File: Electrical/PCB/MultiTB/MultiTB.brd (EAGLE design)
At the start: 9 parts, among them U2 TB6612FNG

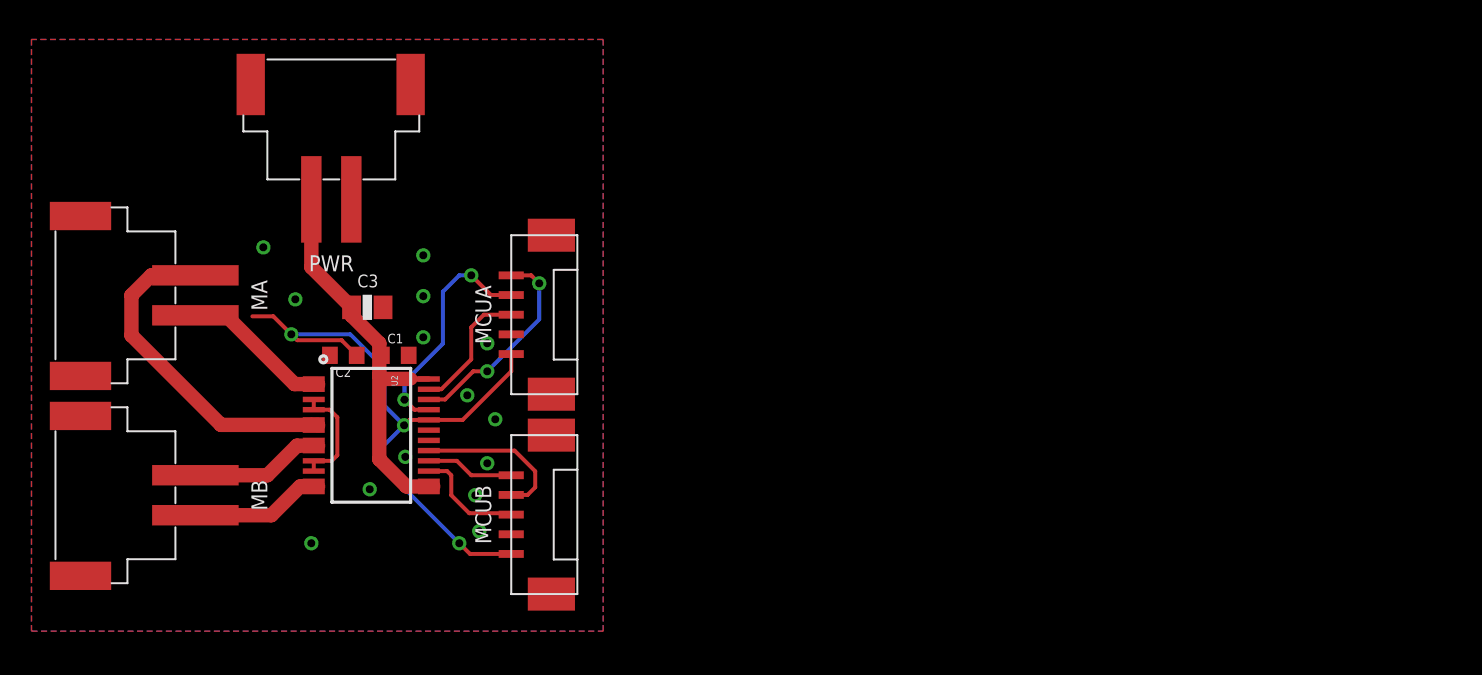
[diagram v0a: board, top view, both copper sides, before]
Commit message: PCB Batch #1
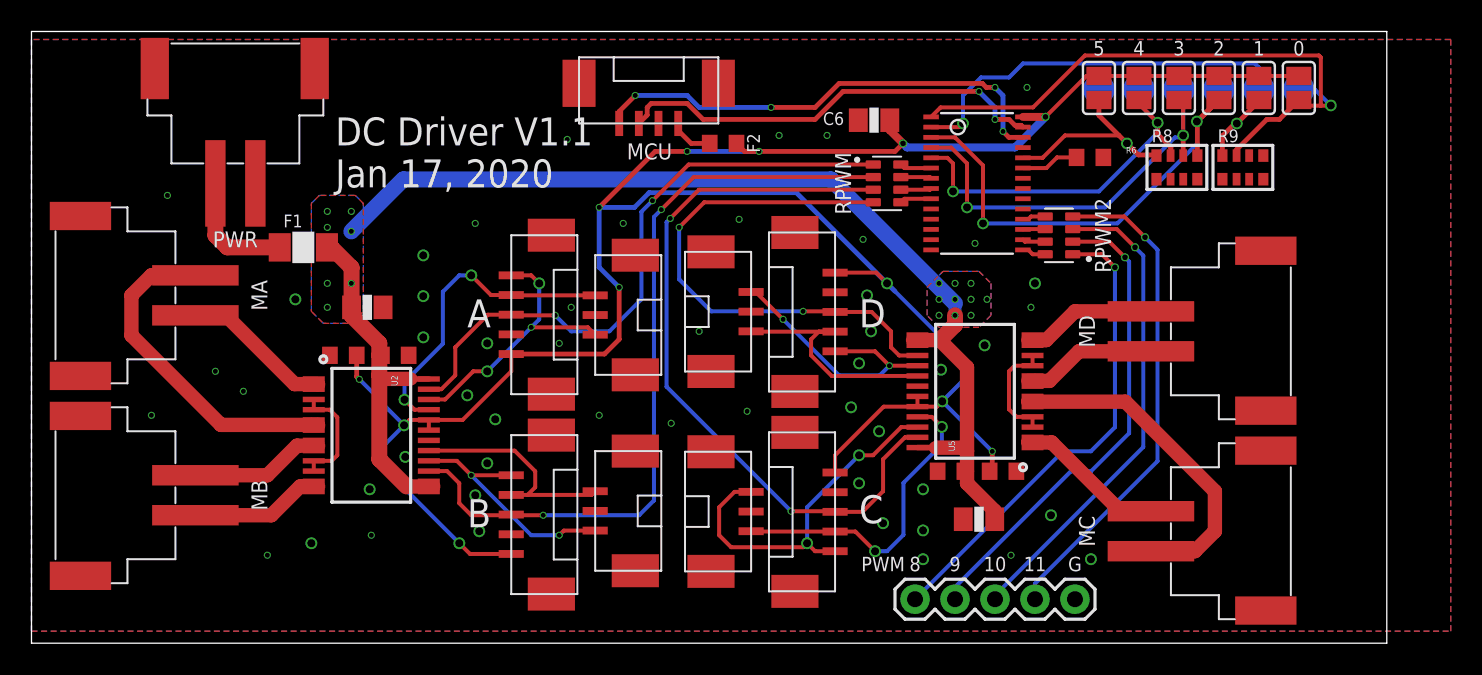
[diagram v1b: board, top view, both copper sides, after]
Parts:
- added C11, C12: 0.1uF, Scott-Electrical:0603
- added C13, C6: 10uF, Scott-Electrical:0805
- added F1: 7A, Scott-Electrical:1206
- added F2: 2A, Scott-Electrical:0603
- added J1: (no value), SparkFun-Connectors:1X05
- added MACTRL, MBCTRL, MCCTRL, MDCTRL: JST_1.25_3P, Scott-Connectors:JST1.25_3P
- added MC, MD: JST_XH_2.54_2P, Scott-Connectors:JST_XH_2.54_2P
- added MCU: JST_1.25_4P, Scott-Connectors:JST1.25_4P
- added MCUC, MCUD: JST_1.25_5P, Scott-Connectors:JST1.25_5P
- added R6: 10K, Scott-Electrical:0603
- added R8, R9: 10K, microbuilder:RESPACK_4X0603
- added RPWM, RPWM2: 330, Scott-Electrical:RESCAF80P320X160X60-8N
- added SJ_A12, SJ_A13, SJ_A14, SJ_A15, SJ_A16, SJ_A17: (no value), microbuilder:SOLDERJUMPER_REFLOW_NOPASTE
- added TP13, TP14, TP15, TP16, TP17, TP18: (no value), microbuilder:TESTPOINT_ROUND_2MM
- added U4: PCA9685, microbuilder:TSSOP28
- added U5: TB6612FNG, SparkFun-IC-Special-Function:SSOP24
- moved PWR 6.18 mm to (1.52, 30.2)
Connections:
- removed net STBY: U2.19
- removed net VCC: C2.1, MCUA.5, MCUB.5, U2.20
- new net 3.3V: C12.1, C2.1, C6.1, F2.1, MCUA.5, MCUB.5, MCUC.5, MCUD.5, SJ_A12.1, SJ_A13.1, SJ_A14.1, SJ_A15.1, SJ_A16.1, SJ_A17.1, U2.19, U2.20, U4.28, U5.19, U5.20
- new net A0: R9.7, SJ_A12.2, TP13.P$1, U4.1
- new net A1: R9.8, SJ_A13.2, TP14.P$1, U4.2
- new net A2: R8.5, SJ_A14.2, TP15.P$1, U4.3
- new net A3: R8.6, SJ_A15.2, TP16.P$1, U4.4
- new net A4: R8.7, SJ_A16.2, TP17.P$1, U4.5
- new net A5: R8.8, SJ_A17.2, TP18.P$1, U4.24
- new net C01: MC.1, U5.1, U5.2
- new net C02: MC.2, U5.5, U5.6
- new net CIN1: MCCTRL.1, MCUC.2, U5.21
- new net CIN2: MCCTRL.3, MCUC.1, U5.22
- new net D01: MD.1, U5.11, U5.12
- new net D02: MD.2, U5.7, U5.8
- new net DIN1: MCUD.2, MDCTRL.1, U5.17
- new net DIN2: MCUD.1, MDCTRL.3, U5.16
- new net N$1: J1.1, RPWM2.1
- new net N$2: F2.2, MCU.4
- new net N$3: J1.2, RPWM2.2
- new net N$4: J1.3, RPWM2.3
- new net N$5: J1.4, RPWM2.4
- new net OE: R6.1, U4.23
- new net PWM0: RPWM.8, U4.6
- new net PWM1: RPWM.7, U4.7
- new net PWM10: RPWM2.6, U4.17
- new net PWM11: RPWM2.5, U4.18
- new net PWM12: U4.19
- new net PWM13: U4.20
- new net PWM14: U4.21
- new net PWM15: U4.22
- new net PWM2: RPWM.6, U4.8
- new net PWM3: RPWM.5, U4.9
- new net PWM4: U4.10
- new net PWM5: U4.11
- new net PWM6: U4.12
- new net PWM7: U4.13
- new net PWM8: RPWM2.8, U4.15
- new net PWM9: RPWM2.7, U4.16
- new net PWMC: MCUC.3, RPWM.3, U5.23
- new net PWMD: MCUD.3, RPWM.4, U5.15
- new net SCL: MCU.1, U4.26
- new net SDA: MCU.2, U4.27
- new net VMIN: F1.1, PWR.1
- net AIN1: now also MACTRL.1
- net AIN2: now also MACTRL.3
- net BIN1: now also MBCTRL.1
- net BIN2: now also MBCTRL.3
- net GND: now also C11.2, C12.2, C13.2, C6.2, J1.5, MACTRL.2, MBCTRL.2, MCCTRL.2, MCU.3, MCUC.4, MCUD.4, MDCTRL.2, R6.2, R8.1, R8.2, R8.3, R8.4, R9.1, R9.2, U4.14, U4.25, U5.10, U5.18, U5.3, U5.4, U5.9
- net PWMA: now also RPWM.1
- net PWMB: now also RPWM.2
- net VM: now also C11.1, C13.1, F1.2, U5.13, U5.14, U5.24; no longer PWR.1
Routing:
- net 3.3V: track 0.00 -> 150.1 mm, vias 0 -> 12
- net VM: track 26.6 -> 87.8 mm, vias 0 -> 17
- net PWMC: track 0.00 -> 46.8 mm, vias 0 -> 2
- net PWMB: track 7.12 -> 49.6 mm, vias 0 -> 2
- net VCC: track 41.8 -> 0.00 mm, vias 3 -> 0
- net A0: track 0.00 -> 40.0 mm, vias 0 -> 1
- net PWMD: track 0.00 -> 34.0 mm, vias 0 -> 2
- net A2: track 0.00 -> 33.5 mm, vias 0 -> 2
- net A1: track 0.00 -> 32.4 mm, vias 0 -> 2
- net N$5: track 0.00 -> 31.7 mm, vias 0 -> 1
- net PWMA: track 8.39 -> 39.3 mm, vias 0 -> 2
- net N$4: track 0.00 -> 30.9 mm, vias 0 -> 1
- net N$3: track 0.00 -> 30.9 mm, vias 0 -> 1
- net SCL: track 0.00 -> 30.5 mm, vias 0 -> 4
- net N$1: track 0.00 -> 30.4 mm, vias 0 -> 1
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- added copper zone on layer 1, net VM
- added copper zone on layer 16, net VM
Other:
- board outline added: 86.1 x 38.9 mm
- board text added: "0"
- board text added: "1"
- board text added: "10"
- board text added: "11"
- board text added: "2"
- board text added: "3"
- board text added: "4"
- board text added: "5"
- board text added: "8"
- board text added: "9"
- board text added: "A"
- board text added: "B"
- board text added: "C"
- board text added: "D"
- board text added: "DC Driver V1.1 Jan 17, 2020"
- board text added: "G"
- board text added: "PWM"
